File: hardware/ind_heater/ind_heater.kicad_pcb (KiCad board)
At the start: 2 copper layers, 95.9 x 47 mm, 18 parts, among them J1 DG126-5.0-02P, J2 Conn_01x01_Male, J3 Conn_01x01_Male, J4 Conn_01x01_Male, Q1 IRFZ46N, Q2 IRFZ46N

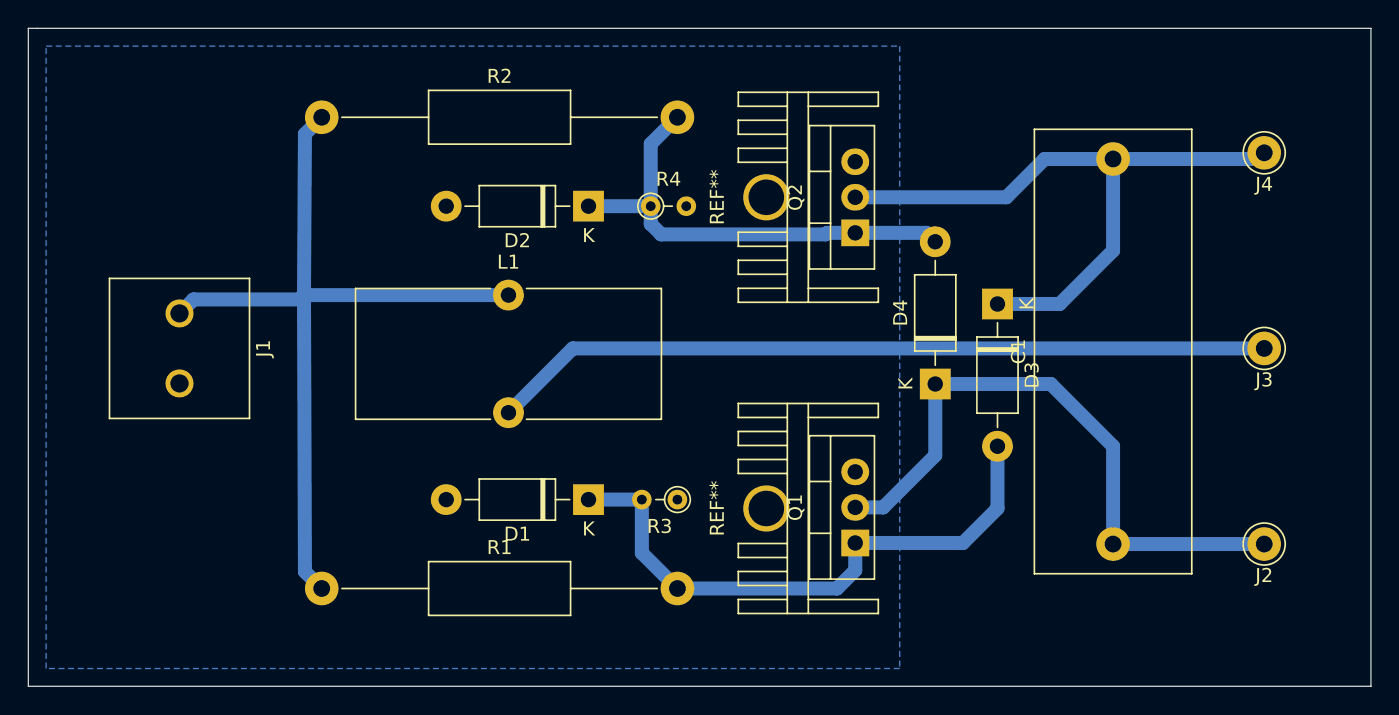
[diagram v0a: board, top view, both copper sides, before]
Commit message: gitignore added
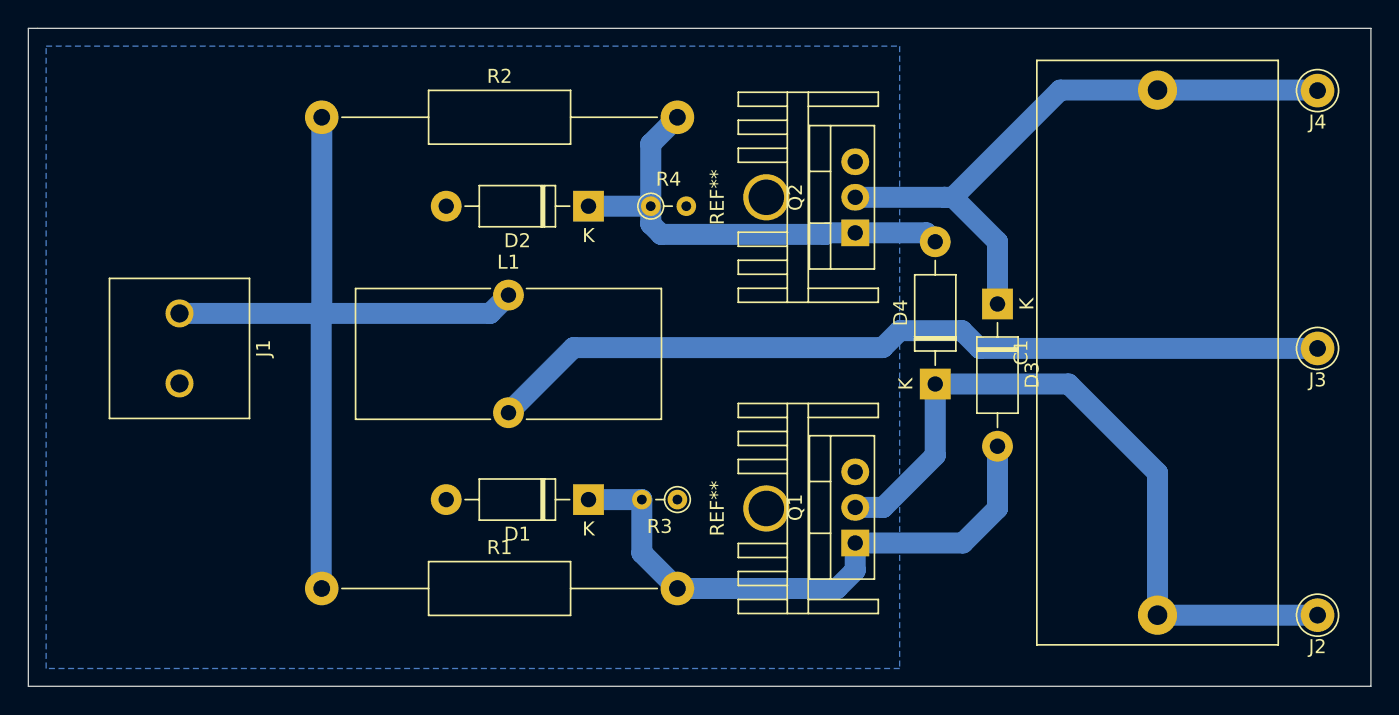
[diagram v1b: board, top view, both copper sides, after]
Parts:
- C1: value C -> 0.47; footprint Capacitor_THT:C_Rect_L31.5mm_W11.0mm_P27.50mm_MKS4 -> Capacitor_THT:C_Rect_L41.5mm_W17.0mm_P37.50mm_MKS4
- moved J2 6.35 mm to (199.4, 128.3)
- moved C1 5.99 mm to (188.0, 128.3)
- moved J4 5.85 mm to (199.4, 90.8)
- moved J3 3.81 mm to (199.4, 109.2)
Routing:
- net Net-(C1-Pad1): track 44.7 -> 52.4 mm
- net Net-(J3-Pad1): track 55.9 -> 60.7 mm
- net Net-(C1-Pad2): track 46.9 -> 45.1 mm
- net +12V: track 58.7 -> 57.7 mm
